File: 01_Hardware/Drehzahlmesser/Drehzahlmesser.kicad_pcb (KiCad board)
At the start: 2 copper layers, 96 x 37 mm, 47 parts, among them J1 Conn_01x02_Female, J2 USB_B_Mini, J3 Conn_01x04_Male, J4 Conn_01x02_Female, SW1 SW_Push, U1 STM32L412K8Tx, U2 LCD_NHD-0108CZ, U3 AP7384, U4 PCF8563T, U5 OPA330xxDBV, Y1 Crystal

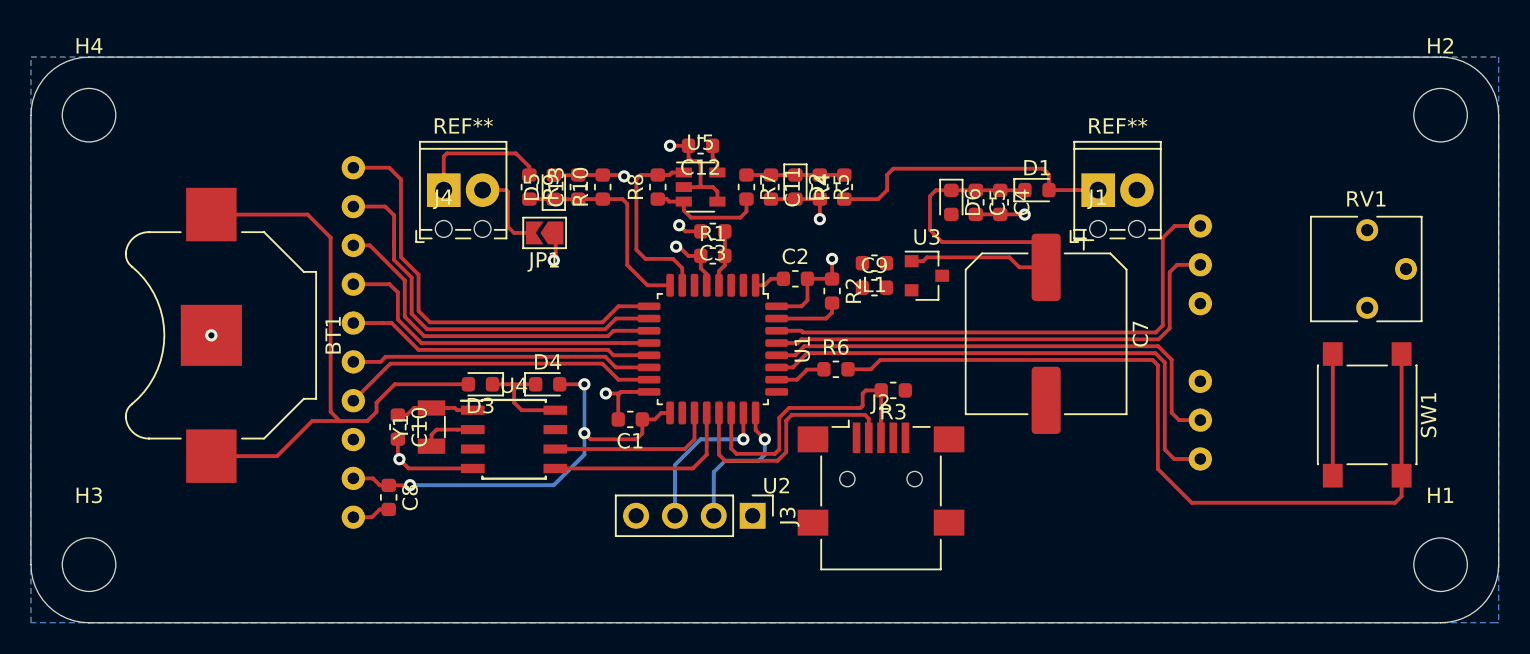
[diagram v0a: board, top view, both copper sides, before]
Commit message: hardware update
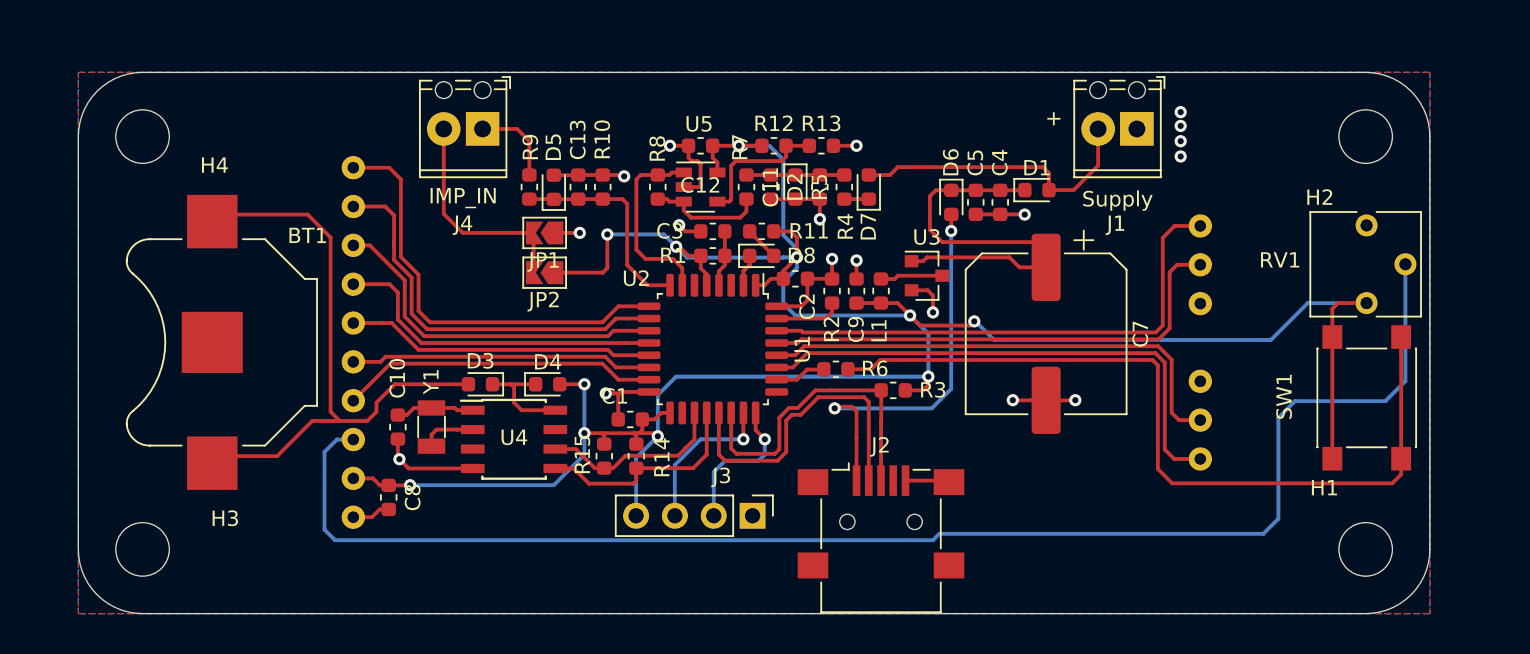
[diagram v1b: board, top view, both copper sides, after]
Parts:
- added D7: D_Schottky, Diode_SMD:D_0603_1608Metric, F.Cu at (141.8, 56.5)
- added D8: LED, LED_SMD:LED_0603_1608Metric, F.Cu at (134.8, 61.0)
- added JP2: JP_VCC, Jumper:SolderJumper-2_P1.3mm_Open_TrianglePad1.0x1.5mm, F.Cu at (120.6, 62.1)
- added R11: 100k, Resistor_SMD:R_0603_1608Metric, F.Cu at (134.8, 59.4)
- added R12: 10k, Resistor_SMD:R_0603_1608Metric, F.Cu at (135.6, 53.8)
- added R13: 10k, Resistor_SMD:R_0603_1608Metric, F.Cu at (138.7, 53.8)
- added R14: 10k, Resistor_SMD:R_0603_1608Metric, F.Cu at (126.6, 74.1)
- added R15: 10k, Resistor_SMD:R_0603_1608Metric, F.Cu at (124.5, 74.1)
- C4: value C -> 10u
- C5: value C -> 1u
- C7: value CP -> 470u
- JP1: value Jumper_NC_Small -> JP_GND
- R7: value R -> 1k
- R8: value R -> 4.7k
- moved H2 5.10 mm to (174.3, 53.2)
- moved H1 5.00 mm to (174.3, 80.2)
- moved J4 4.74 mm to (116.5, 52.7), turned to 180 degrees
- moved J1 4.74 mm to (159.3, 52.7), turned to 180 degrees
- moved H4 3.77 mm to (94.3, 53.2)
- moved H3 3.64 mm to (94.3, 80.2)
- moved J2 2.80 mm to (142.6, 78.4)
- moved L1 1.87 mm to (142.6, 63.3), turned to 270 degrees
- moved C9 1.19 mm to (141.0, 63.3), turned to 90 degrees
- moved SW1 1.11 mm to (174.4, 70.3)
- moved BT1 0.46 mm to (98.9, 66.7)
- moved RV1 0.31 mm to (174.4, 64.1)
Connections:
- J1 pad 1: AC -> GND
- J1 pad 2: GND -> AC
- J2 pad 4: Net-(J2-Pad4) -> (no net)
- J3 pad 1: +3V3 -> GND
- J3 pad 4: GND -> +3V3
- R4 pad 1: AC -> Net-(D7-Pad1)
- U1 pad 18: Net-(U1-Pad18) -> (no net)
- U1 pad 2: Net-(U1-Pad2) -> LED
- U1 pad 25: Net-(U1-Pad25) -> (no net)
- U1 pad 3: Net-(U1-Pad3) -> (no net)
- U1 pad 6: Net-(U1-Pad6) -> (no net)
- U2 pad 15: Net-(U2-Pad15) -> (no net)
- U2 pad 16: Net-(U2-Pad16) -> (no net)
- U4 pad 3: Net-(U4-Pad3) -> (no net)
- U4 pad 7: Net-(U4-Pad7) -> (no net)
- U5 pad 4: GND -> Net-(R12-Pad2)
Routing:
- net +3V3: track 45.1 -> 169.7 mm, vias 4 -> 11
- net Net-(RV1-Pad2): track 0.00 -> 94.1 mm
- net VBUS: track 0.00 -> 25.7 mm, vias 0 -> 2
- net GND: track 43.5 -> 53.6 mm, vias 10 -> 18
- net Net-(R12-Pad2): track 0.00 -> 9.25 mm
- net Net-(J4-Pad2): track 5.84 -> 14.5 mm
- net D-: track 16.5 -> 20.9 mm
- net Net-(L1-Pad1): track 0.00 -> 4.09 mm
- net Net-(J4-Pad1): track 8.78 -> 5.60 mm
- net D+: track 18.8 -> 21.1 mm
- net Net-(D8-Pad2): track 0.00 -> 2.25 mm
- net LED: track 0.00 -> 2.10 mm
- net Net-(D7-Pad1): track 0.00 -> 1.60 mm
- net SDA: track 13.0 -> 14.3 mm
- net SCL: track 11.1 -> 12.2 mm
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- added copper zone on F.Cu, net GND
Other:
- board size 96 x 37 mm -> 88.4 x 35.4 mm
- board text added: "+"
